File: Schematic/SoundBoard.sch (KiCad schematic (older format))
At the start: 0 parts

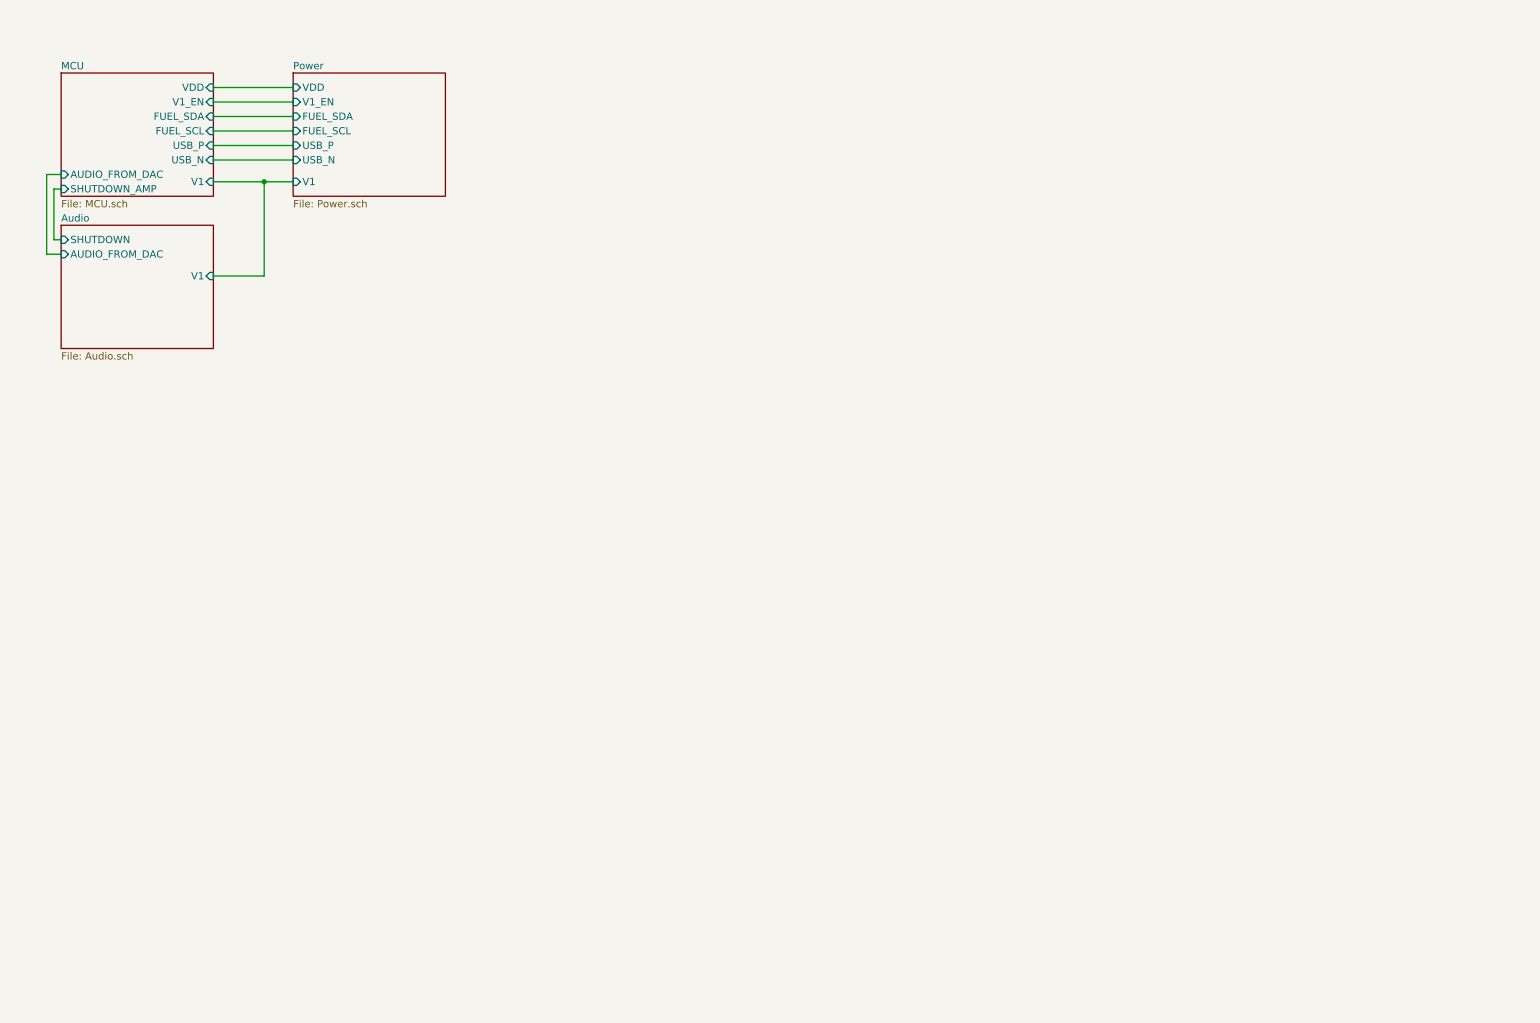
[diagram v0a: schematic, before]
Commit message: Inital rev 1.0 commit
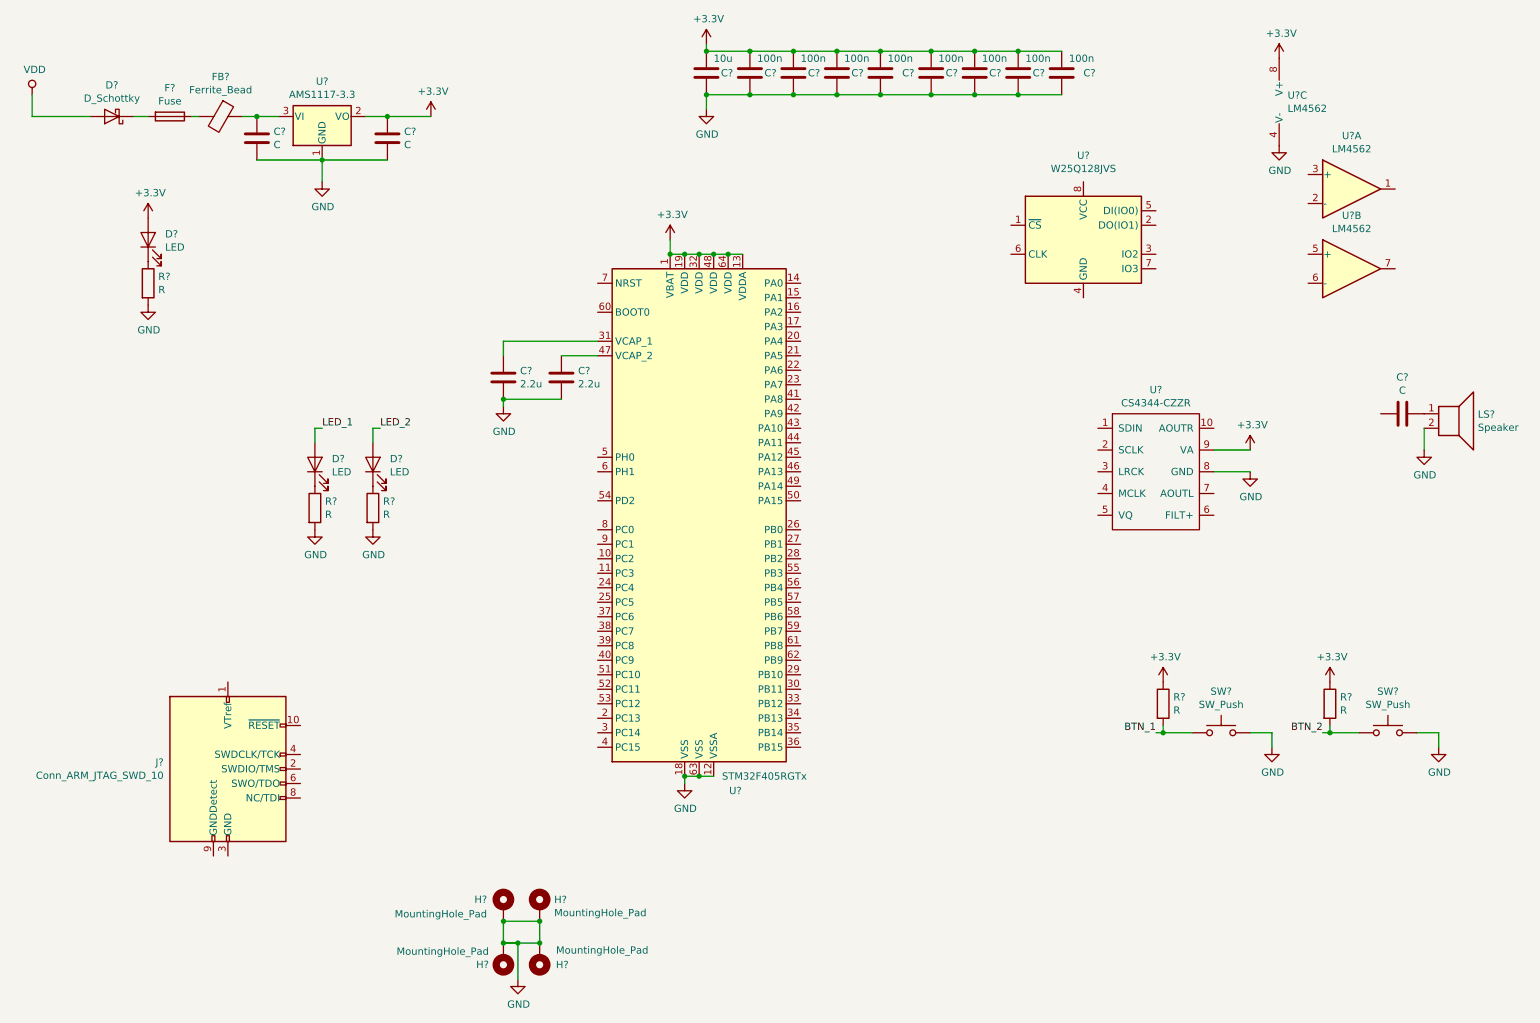
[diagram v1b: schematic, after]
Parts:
- added C? (x8): 100n, symbol Device:C
- added C?: 10u, symbol Device:C
- added C? (x3): C, symbol Device:C
- added C? (x2): 2.2u, symbol Device:C
- added D?: D_Schottky, symbol Device:D_Schottky
- added D? (x3): LED, symbol Device:LED
- added F?: Fuse, symbol Device:Fuse
- added FB?: Ferrite_Bead, symbol Device:Ferrite_Bead
- added H? (x4): MountingHole_Pad, symbol Mechanical:MountingHole_Pad
- added J?: Conn_ARM_JTAG_SWD_10, symbol Connector:Conn_ARM_JTAG_SWD_10
- added LS?: Speaker, symbol Device:Speaker
- added R? (x5): R, symbol Device:R
- added SW? (x2): SW_Push, symbol Switch:SW_Push
- added U?: STM32F405RGTx, Package_QFP:LQFP-64_10x10mm_P0.5mm, symbol MCU_ST_STM32F4:STM32F405RGTx
- added U?: AMS1117-3.3, Package_TO_SOT_SMD:SOT-223-3_TabPin2, symbol Regulator_Linear:AMS1117-3.3
- added U? (x3): LM4562, symbol Amplifier_Operational:LM4562
- added U?: CS4344-CZZR, symbol SoundBoard:CS4344-CZZR
- added U?: W25Q128JVS, Package_SO:SOIC-8_5.23x5.23mm_P1.27mm, symbol Memory_Flash:W25Q128JVS
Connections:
- new net: C?.1, U?.31 (VCAP_1)
- new net: C?.1, U?.47 (VCAP_2)
- new net: C?.1, FB?.1, U?.3 (VI)
- new net: D?.1 (K), F?.2
- new net: F?.1, FB?.2
- new net: C?.1, LS?.1
- new net: D?.1 (K), R?.1 (x3)
- new net: J?.3 (GND), J?.5 (GND)
- new net +3V3: C?.1, C?.1, C?.1, C?.1, C?.1, C?.1, C?.1, C?.1, C?.1, C?.1, D?.2 (A), R?.1, R?.1, U?.1 (VBAT), U?.13 (VDDA), U?.19 (VDD), U?.2 (VO), U?.32 (VDD), U?.48 (VDD), U?.64 (VDD), U?.8 (V+), U?.9 (VA)
- new net BTN_1: R?.2, SW?.1
- new net BTN_2: R?.2, SW?.1
- new net GND: C?.2, C?.2, C?.2, C?.2, C?.2, C?.2, C?.2, C?.2, C?.2, C?.2, C?.2, C?.2, C?.2, H?.1, H?.1, H?.1, H?.1, LS?.2, R?.2, R?.2, R?.2, SW?.2, SW?.2, U?.1 (GND), U?.12 (VSSA), U?.18 (VSS), U?.4 (V-), U?.63 (VSS), U?.8 (GND)
- new net LED_1: D?.2 (A)
- new net LED_2: D?.2 (A)
- new net VDD: D?.2 (A)
